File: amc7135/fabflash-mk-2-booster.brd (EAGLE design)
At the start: 30 x 16 mm, 15 parts, among them U1 LM2735YMF

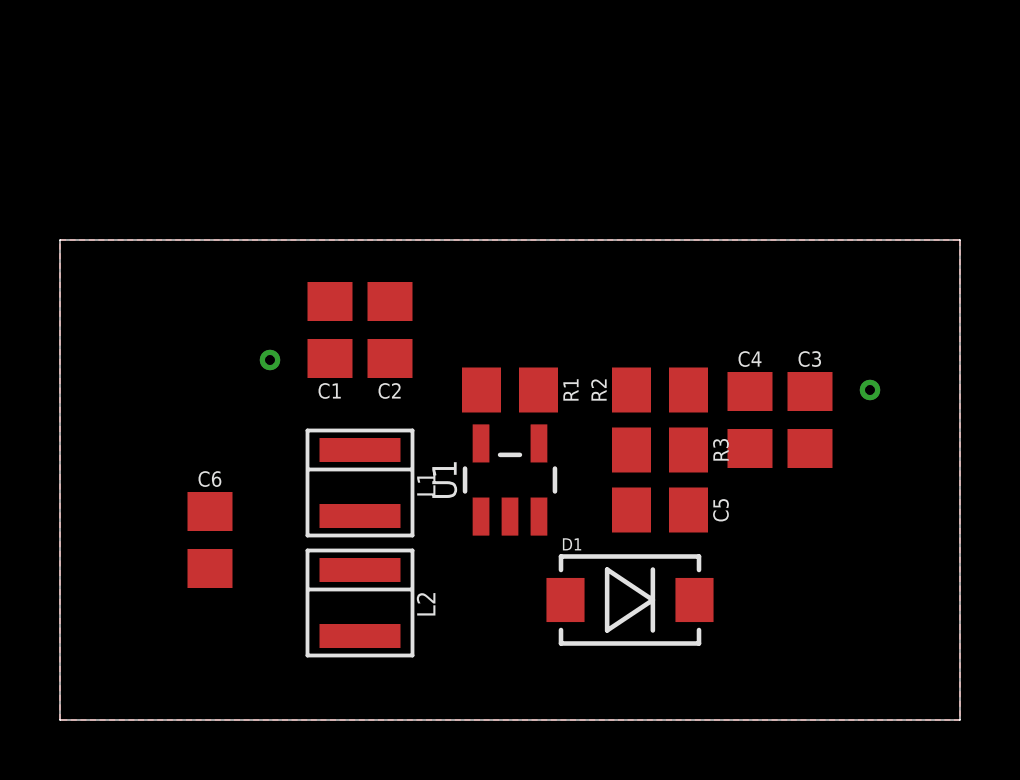
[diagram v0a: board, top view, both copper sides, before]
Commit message: faaaabulous flashlight in progress
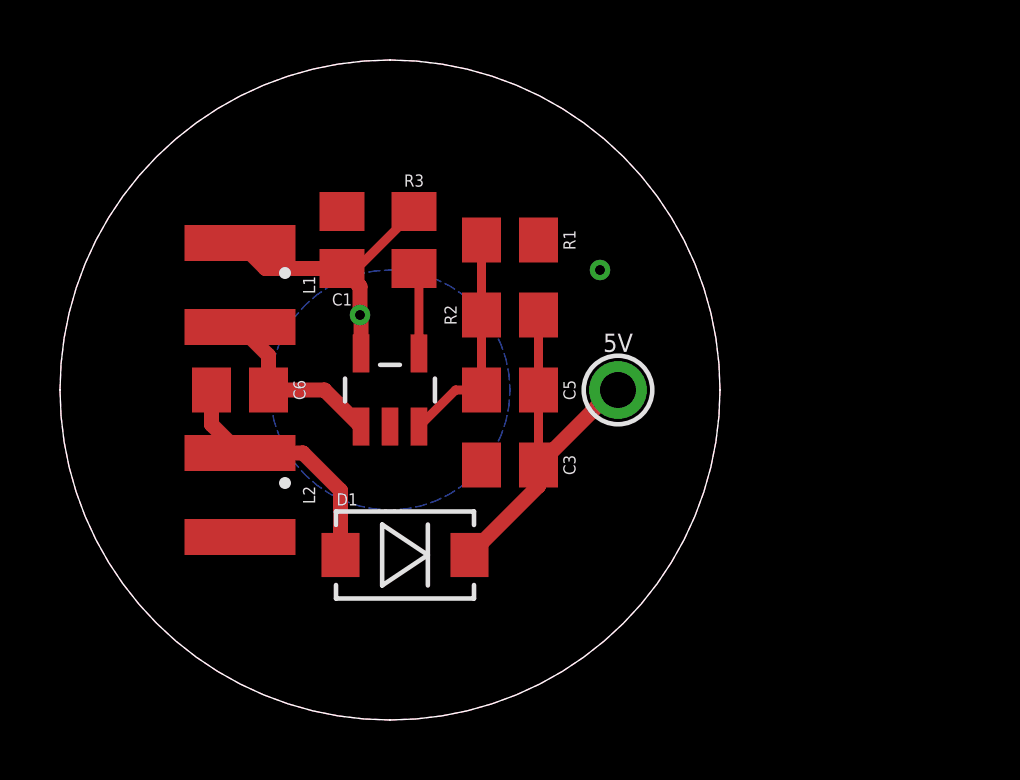
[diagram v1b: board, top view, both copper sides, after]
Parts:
- removed C2, C4: (no value), A_butts:C0805
- removed JP1, JP2: M01NOT-A-VIA-NOPE, A_butts:1X01_NOSILK_NOSTOP
- added 5V: M01PTH-1.2MM, A_butts:1X01-1.2MM
- added BATT+, BATT-: M01NOT-A-VIA-NOPE, A_butts:1X01_NOSILK_NOSTOP
- C1: value (none) -> 22uF
- C3: value (none) -> 10uF
- C5: value (none) -> 2.2nF
- C6: value (none) -> 2.2uF
- L1, L2: device A_butts:TAIYO-YUDEN-30XX -> A_butts:TAIYO-YUDEN-40XX
- R1: value (none) -> 10k
- R2: value (none) -> 30k
- R3: value (none) -> 100k
- moved R3 10.8 mm to (11.8, 16.0), turned to 270 degrees
- moved C3 10.1 mm to (15.0, 8.50), turned to 180 degrees
- moved D1 7.65 mm to (11.5, 5.50)
- moved L1 6.80 mm to (6.00, 14.5)
- moved C5 6.40 mm to (15.0, 11.0)
- moved R2 5.59 mm to (15.0, 13.5)
- moved C6 5.10 mm to (6.00, 11.0), turned to 180 degrees
- moved R1 5.00 mm to (15.0, 16.0)
- moved U1 5.00 mm to (11.0, 11.0)
- moved L2 4.72 mm to (6.00, 7.50)
- moved C1 3.03 mm to (9.40, 16.0)
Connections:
- net GND: now also BATT-.P$1, R1.1; no longer C4.2, R3.1
- net N$2: now also R3.2; no longer R1.1
- net N$8: now also R1.2; no longer R3.2
- net VIN: now also BATT+.P$1, R3.1; no longer C2.1, JP1.P$1, R1.2
- net VOUT: now also 5V.P$1; no longer C4.1, JP2.P$1
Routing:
- net VOUT: track 0.00 -> 12.6 mm
- net VIN: track 0.00 -> 10.1 mm
- net N$6: track 0.00 -> 8.51 mm
- net N$8: track 0.00 -> 7.59 mm
- net N$1: track 0.00 -> 6.08 mm
- net N$2: track 0.00 -> 2.88 mm
- added copper zone on layer 16, net GND
- added copper zone on layer 16, net VIN
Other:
- board size 30 x 16 mm -> 22 x 22 mm
